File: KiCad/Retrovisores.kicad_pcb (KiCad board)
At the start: 2 copper layers, 68 parts, among them J1 Conn_01x02_Pin, J10 Conn_01x07_Pin, J11 Conn_01x02_Pin, J2 DE9_Pins, J3 Conn_01x04_Pin, J4 DE9_Pins, J5 Conn_01x02_Pin, J6 Conn_01x02_Pin, J7 Conn_01x02_Pin, J8 Conn_PIC_ICSP_ICD, J9 Conn_01x04_Pin, K2 Relay_SPDT, Q14 AO3400A, Q15 AO3401A, Q16 AO3400A, Q17 AO3401A, Q18 AO3400A, Q19 AO3401A, Q20 AO3400A, Q21 AO3401A, Q22 AO3400A, Q23 AO3401A, Q24 AO3400A, Q25 AO3401A, Q27 AO3400A, SW1 SW_Push, SW2 SW_Push, SW3 SW_Push, SW4 SW_Push, SW6 SW_Nidec_CAS-120A1, U2 SN65HVD232, U4 LT1117-3.3, U5 TSR3-2450N, U7 PIC32MX250F128D-IPT, Y1 Crystal

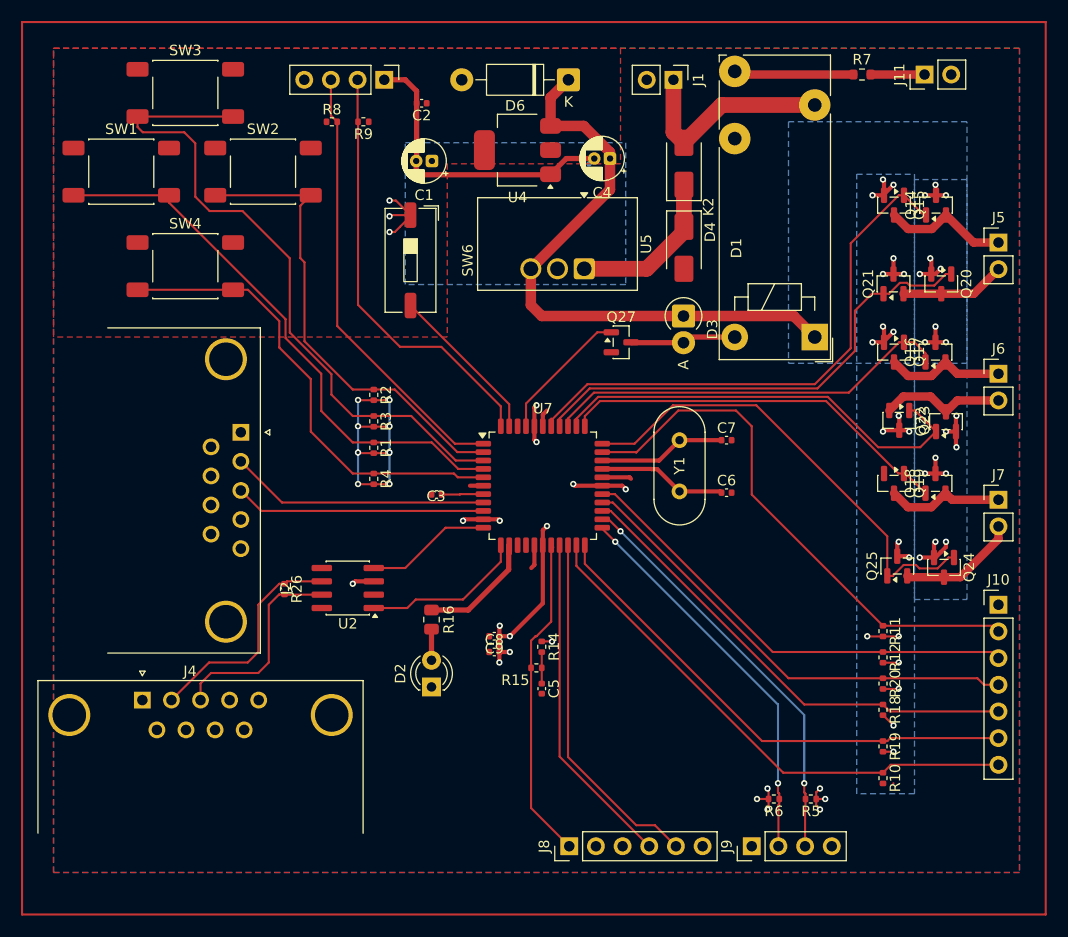
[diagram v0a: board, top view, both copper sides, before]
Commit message: versión casi final del enrutado
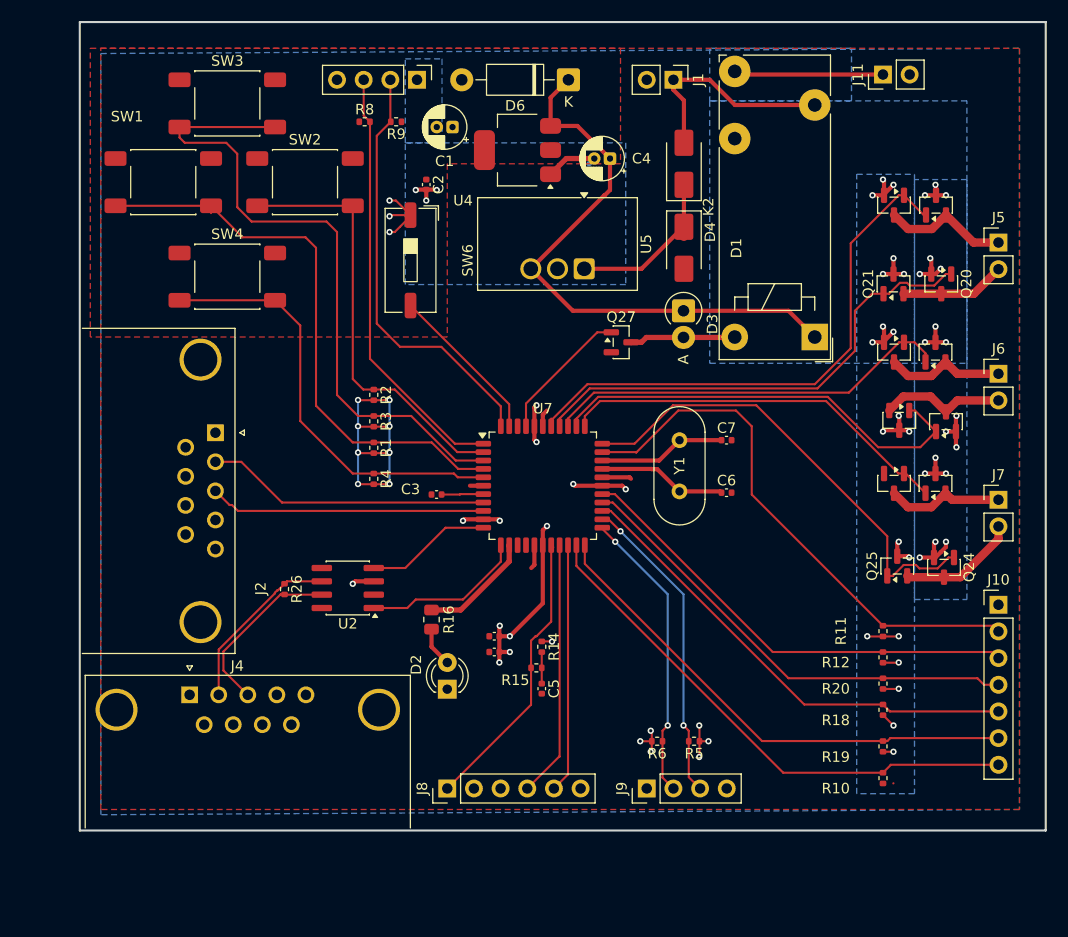
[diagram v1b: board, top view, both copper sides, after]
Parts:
- removed R7: 4.7k, Resistor_SMD:R_0603_1608Metric
- moved J8 12.9 mm to (125.5, 98.0)
- moved R5 12.4 mm to (149.0, 93.5)
- moved R6 12.4 mm to (145.5, 93.5)
- moved J9 11.4 mm to (144.5, 98.0)
- moved C2 7.76 mm to (123.5, 40.5), turned to -90 degrees
- moved J4 4.53 mm to (101.0, 89.1)
- moved SW1 4.12 mm to (98.5, 40.2)
- moved SW2 4.12 mm to (112.0, 40.2)
- moved SW3 4.12 mm to (104.5, 32.8)
- moved SW4 4.12 mm to (104.5, 49.2)
- moved J11 3.96 mm to (167.0, 30.0)
- moved C1 3.78 mm to (126.0, 35.0)
- moved J3 3.12 mm to (122.6, 30.5)
- moved R8 3.12 mm to (117.6, 34.5)
- moved R9 3.12 mm to (120.6, 34.5)
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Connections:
- net Net-(U2-CANH) renamed CAN_+
- net Net-(U2-CANL) renamed CAN_-
- K2 pad 14: Net-(K2-Pad14) -> Net-(J11-Pin_1)
- Q14 pad 3: 5V -> VBAT
- Q16 pad 3: 5V -> VBAT
- Q18 pad 3: 5V -> VBAT
- Q20 pad 2: 5V -> VBAT
- Q22 pad 2: 5V -> VBAT
- Q24 pad 2: 5V -> VBAT
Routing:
- net 5V: track 80.6 -> 55.5 mm, vias 18 -> 0
- net VBAT: track 20.4 -> 44.1 mm, vias 0 -> 18
- net GND: track 92.3 -> 71.4 mm, vias 28 -> 31
- net Net-(K2-Pad14): track 11.4 -> 0.00 mm
- net PGC: track 34.0 -> 23.7 mm
- net SCL: track 39.5 -> 29.8 mm
- net SDA: track 37.4 -> 28.1 mm
- net Net-(J11-Pin_1): track 5.14 -> 14.2 mm
- net PGD: track 32.2 -> 24.5 mm
- net CAN_-: track 21.6 -> 16.9 mm
- net L: track 45.0 -> 40.9 mm
- net MCLR: track 31.3 -> 27.6 mm
- net D: track 44.7 -> 41.3 mm
- net CAN_+: track 19.9 -> 16.7 mm
- net RX: track 24.7 -> 27.1 mm
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- added copper zone on B.Cu, net VBAT
- removed copper zone on B.Cu, net 5V
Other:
- board outline added: 92 x 77 mm
